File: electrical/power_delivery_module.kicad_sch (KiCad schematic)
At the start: 8 parts, among them U2 UA78L05AI

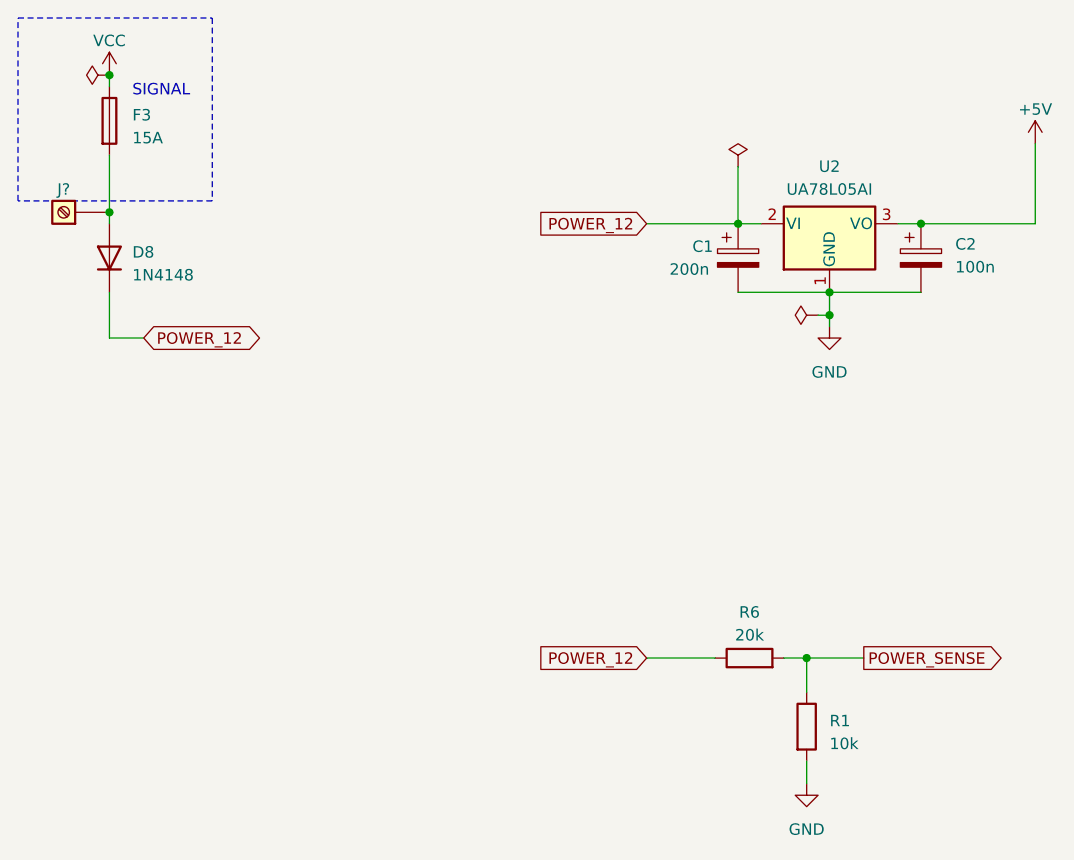
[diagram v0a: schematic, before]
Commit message: Work in progress
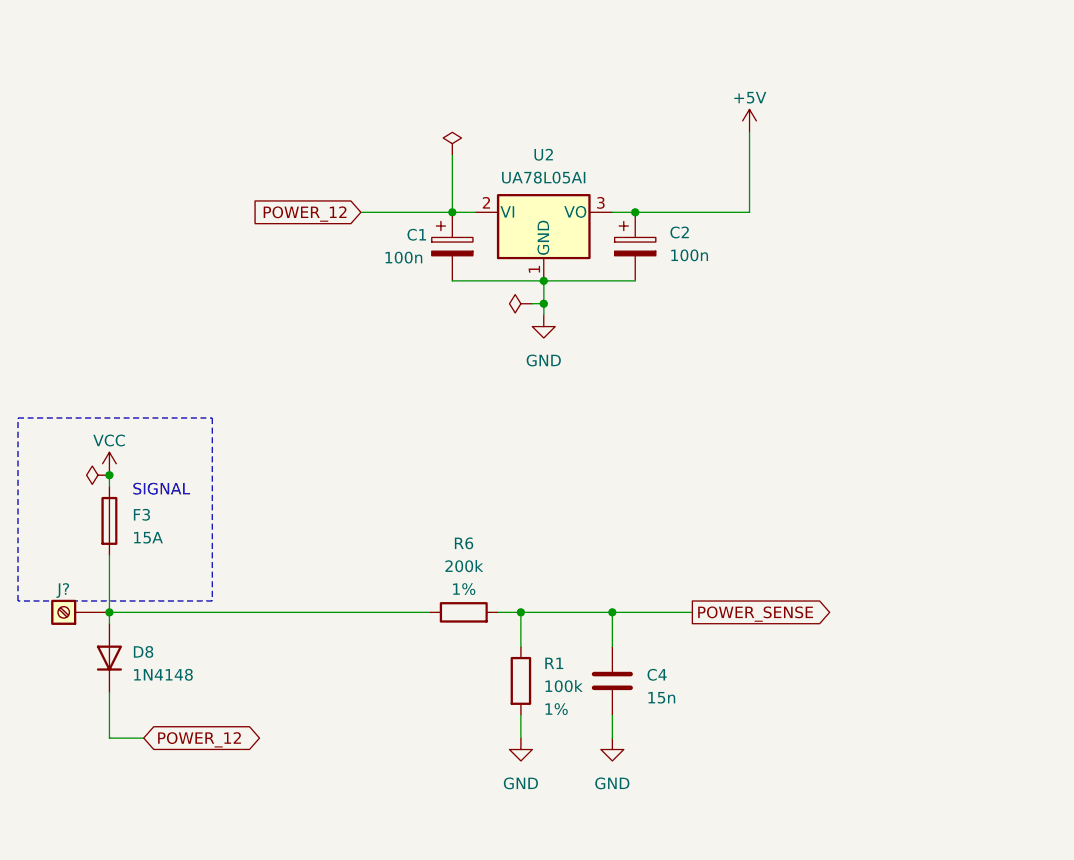
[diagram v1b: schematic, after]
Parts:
- added C4: 15n, symbol Device:C
- C1: value 200n -> 100n
- R1: value 10k -> 100k; Tolerance (none) -> 1%
- R6: value 20k -> 200k; Tolerance (none) -> 1%
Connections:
- net GND: now also C4.2
- net POWER_12: no longer R6.1
- net POWER_SENSE: now also C4.1
- net at D8.2 (A), F3.2, J?.1 (Pin_1): now also R6.1
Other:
- moved on the sheet: C1, C2, D8, F3, J?, R1, R6, U2
